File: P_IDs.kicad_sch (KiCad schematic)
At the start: 1 part

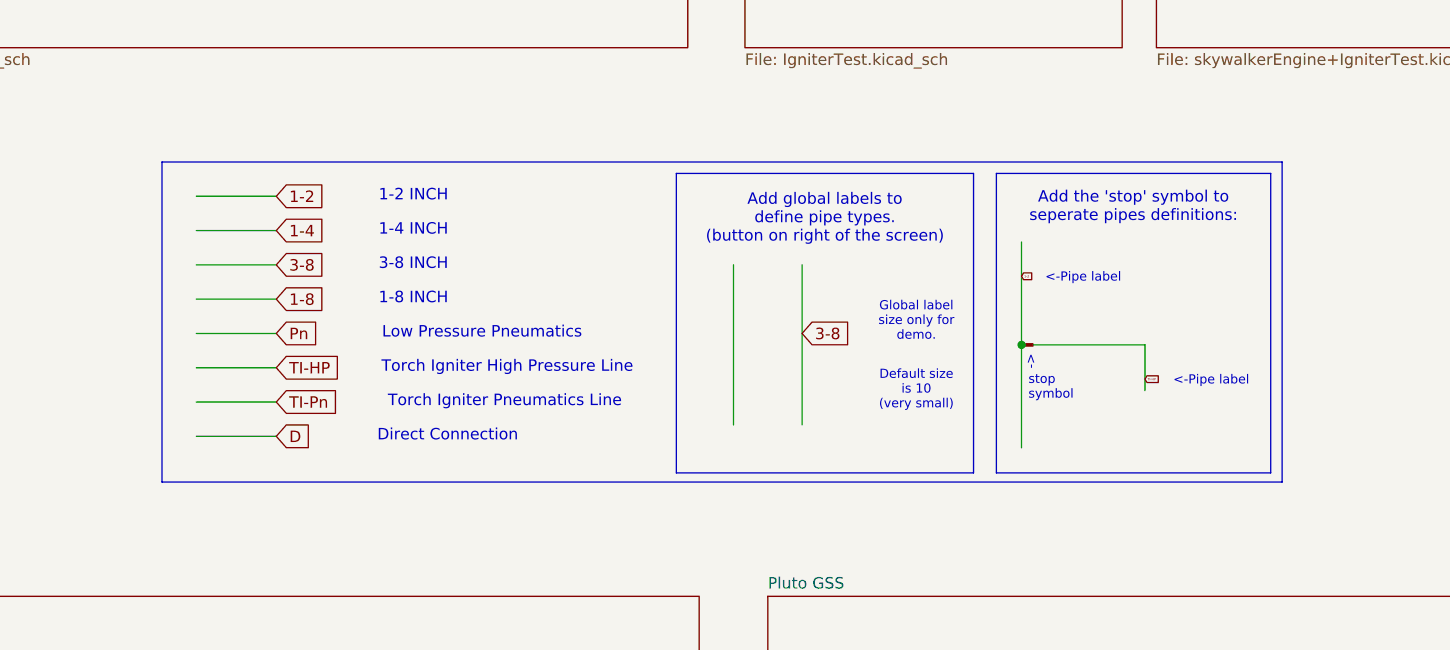
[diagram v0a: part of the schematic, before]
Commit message: bored
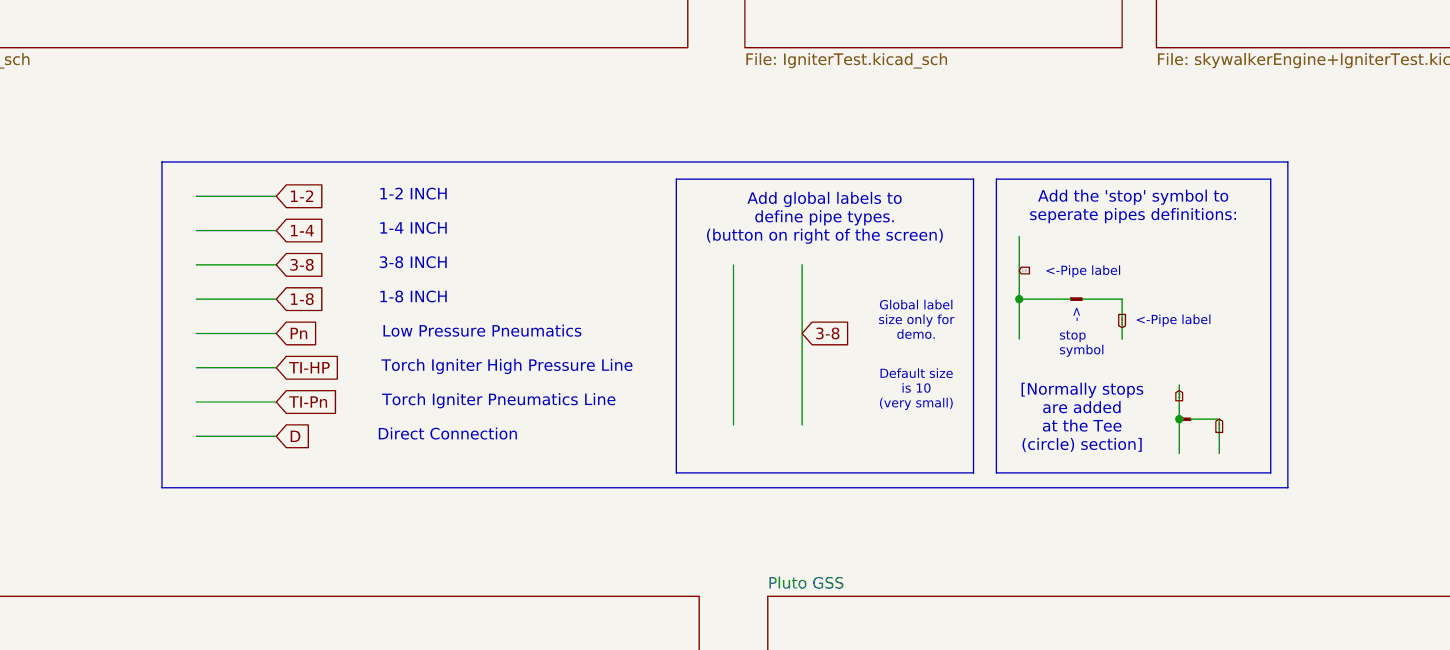
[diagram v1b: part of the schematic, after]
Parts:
- added U11: ~, symbol PID_symbols:stop
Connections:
- net 1-2: now also U11.
- net TI-HP: now also U11.
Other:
- note added: "[Normally stops are added at the Tee (circle) section]"
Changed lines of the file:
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@@
 	(rectangle
 		(start 62.23 86.36)
-		(end 186.69 121.92)
+		(end 187.325 122.555)
 		(stroke
 			(width 0)
@@
 	)
 	(rectangle
-		(start 154.94 87.63)
+		(start 154.94 88.265)
 		(end 185.42 120.904)
 		(stroke
@@
 	)
 	(rectangle
-		(start 119.38 87.63)
+		(start 119.38 88.265)
 		(end 152.4 120.904)
 		(stroke
@@
 	(text "<-Pipe label\n"
 		(exclude_from_sim no)
-		(at 164.592 99.314 0)
+		(at 164.592 98.679 0)
 		(effects
 			(font
@@
 	(text "stop\nsymbol"
 		(exclude_from_sim no)
-		(at 158.496 111.506 0)
+		(at 161.925 106.68 0)
 		(effects
 			(font
@@
 	(text "<-Pipe label\n"
 		(exclude_from_sim no)
-		(at 178.816 110.744 0)
+		(at 174.625 104.14 0)
 		(effects
 			(font
@@
 	(text "Torch Igniter Pneumatics Line"
 		(exclude_from_sim no)
-		(at 100.33 113.03 0)
+		(at 99.695 113.03 0)
 		(effects
 			(font
@@
 		)
 	)
+	(text "[Normally stops \nare added\nat the Tee \n(circle) section]"
+		(exclude_from_sim no)
+		(at 164.465 114.935 0)
+		(effects
+			(font
+				(size 1.27 1.27)
+				(color 204 102 0 1)
+			)
+		)
+	)
 	(text "->"
 		(exclude_from_sim no)
-		(at 158.75 108.712 90)
+		(at 163.83 103.505 90)
 		(effects
 			(font
@@
 	)
 	(junction
-		(at 157.734 106.68)
+		(at 157.48 101.6)
 		(diameter 0)
 		(color 0 0 0 0)
 	)
-	(wire
-		(pts
-			(xy 159.004 106.68) (xy 171.45 106.68)
-		)
-		(stroke
-			(width 0)
-			(type default)
-		)
+	(junction
+		(at 175.26 114.935)
+		(diameter 0)
+		(color 0 0 0 0)
 	)
 	(wire
@@
 	(wire
 		(pts
-			(xy 157.734 95.25) (xy 157.734 106.68)
+			(xy 175.26 111.125) (xy 175.26 114.935)
+		)
+		(stroke
+			(width 0)
+			(type default)
+		)
+	)
+	(wire
+		(pts
+			(xy 175.26 114.935) (xy 175.26 118.745)
+		)
+		(stroke
+			(width 0)
+			(type default)
+		)
+	)
+	(wire
+		(pts
+			(xy 157.48 94.615) (xy 157.48 101.6)
+		)
+		(stroke
+			(width 0)
+			(type default)
+		)
+	)
+	(wire
+		(pts
+			(xy 157.48 101.6) (xy 163.195 101.6)
 		)
 		(stroke
@@
 	(wire
 		(pts
+			(xy 157.48 101.6) (xy 157.48 106.045)
+		)
+		(stroke
+			(width 0)
+			(type default)
+		)
+	)
+	(wire
+		(pts
 			(xy 66.04 109.22) (xy 74.93 109.22)
 		)
@@
 	(wire
 		(pts
+			(xy 179.705 114.935) (xy 179.705 118.745)
+		)
+		(stroke
+			(width 0)
+			(type default)
+		)
+	)
+	(wire
+		(pts
 			(xy 66.04 93.98) (xy 74.93 93.98)
 		)
@@
 	(wire
 		(pts
-			(xy 157.734 106.68) (xy 157.734 118.11)
+			(xy 164.465 101.6) (xy 168.91 101.6)
 		)
 		(stroke
@@
 	(wire
 		(pts
-			(xy 171.45 106.68) (xy 171.45 111.76)
+			(xy 168.91 101.6) (xy 168.91 106.045)
+		)
+		(stroke
+			(width 0)
+			(type default)
+		)
+	)
+	(wire
+		(pts
+			(xy 176.53 114.935) (xy 179.705 114.935)
 		)
 		(stroke
@@
 		)
 	)
+	(global_label "TI-HP"
+		(shape input)
+		(at 179.705 114.935 270)
+		(fields_autoplaced yes)
+		(effects
+			(font
+				(size 0.254 0.254)
+			)
+			(justify right)
+		)
+		(property "Intersheetrefs" "${INTERSHEET_REFS}"
+			(at 179.705 116.6817 90)
+			(effects
+				(font
+					(size 1.27 1.27)
+				)
+				(justify right)
+				(hide yes)
+			)
+		)
+	)
 	(global_label "3-8"
 		(shape input)
@@
 	(global_label "1-2"
 		(shape input)
-		(at 157.734 99.06 0)
+		(at 157.48 98.425 0)
 		(fields_autoplaced yes)
 		(effects
@@
 		)
 		(property "Intersheetrefs" "${INTERSHEET_REFS}"
-			(at 159.1299 99.06 0)
-			(effects
-				(font
-					(size 1.27 1.27)
-				)
-				(justify left)
+			(at 158.8759 98.425 0)
+			(effects
+				(font
+					(size 1.27 1.27)
+				)
+				(justify left)
+				(hide yes)
+			)
+		)
+	)
+	(global_label "1-2"
+		(shape input)
+		(at 175.26 111.76 270)
+		(fields_autoplaced yes)
+		(effects
+			(font
+				(size 0.254 0.254)
+			)
+			(justify right)
+		)
+		(property "Intersheetrefs" "${INTERSHEET_REFS}"
+			(at 175.26 113.1559 90)
+			(effects
+				(font
+					(size 1.27 1.27)
+				)
+				(justify right)
 				(hide yes)
 			)
@@
 	(global_label "TI-HP"
 		(shape input)
-		(at 171.45 110.49 0)
+		(at 168.91 104.775 90)
 		(fields_autoplaced yes)
 		(effects
@@
 		)
 		(property "Intersheetrefs" "${INTERSHEET_REFS}"
-			(at 173.1967 110.49 0)
+			(at 168.91 103.0283 90)
 			(effects
 				(font
@@
 	(symbol
 		(lib_id "PID_symbols:stop")
-		(at 159.004 106.68 0)
+		(at 164.465 101.6 0)
 		(unit 1)
 		(exclude_from_sim no)
@@
 		(fields_autoplaced yes)
 		(property "Reference" "U6"
-			(at 161.29 106.172 0)
+			(at 166.751 101.092 0)
 			(effects
 				(font
@@
 		)
 		(property "Value" "~"
-			(at 158.369 105.41 0)
+			(at 163.83 100.33 0)
 			(effects
 				(font
@@
 		)
 		(property "Footprint" ""
-			(at 159.004 106.68 0)
+			(at 164.465 101.6 0)
 			(effects
 				(font
@@
 		)
 		(property "Datasheet" ""
-			(at 159.004 106.68 0)
+			(at 164.465 101.6 0)
 			(effects
 				(font
@@
 		)
 		(property "Description" ""
-			(at 159.004 106.68 0)
+			(at 164.465 101.6 0)
 			(effects
 				(font
@@
 					(unit 1)
 				)
+			)
+		)
+	)
+	(symbol
+		(lib_name "stop_1")
+		(lib_id "PID_symbols:stop")
+		(at 176.53 114.935 0)
+		(unit 1)
+		(exclude_from_sim no)
+		(in_bom no)
+		(on_board no)
+		(dnp no)
+		(fields_autoplaced yes)
+		(property "Reference" "U11"
+			(at 178.816 114.427 0)
+			(effects
+				(font
+					(size 1.27 1.27)
+				)
+				(hide yes)
+			)
+		)
+		(property "Value" "~"
+			(at 175.895 113.665 0)
+			(effects
+				(font
+					(size 1.27 1.27)
+				)
+			)
+		)
+		(property "Footprint" ""
+			(at 176.53 114.935 0)
+			(effects
+				(font
+					(size 1.27 1.27)
+				)
+				(hide yes)
+			)
+		)
+		(property "Datasheet" ""
+			(at 176.53 114.935 0)
+			(effects
+				(font
+					(size 1.27 1.27)
+				)
+				(hide yes)
+			)
+		)
+		(property "Description" ""
+			(at 176.53 114.935 0)
+			(effects
+				(font
+					(size 1.27 1.27)
+				)
+				(hide yes)
+			)
+		)
+		(pin ""
+		)
+		(pin ""
+		)
+		(instances
+			(project ""
+				(path "/045f1f05-3134-4b6d-91b6-463031104f1e"
+					(reference "U11")
+					(unit 1)
+				)

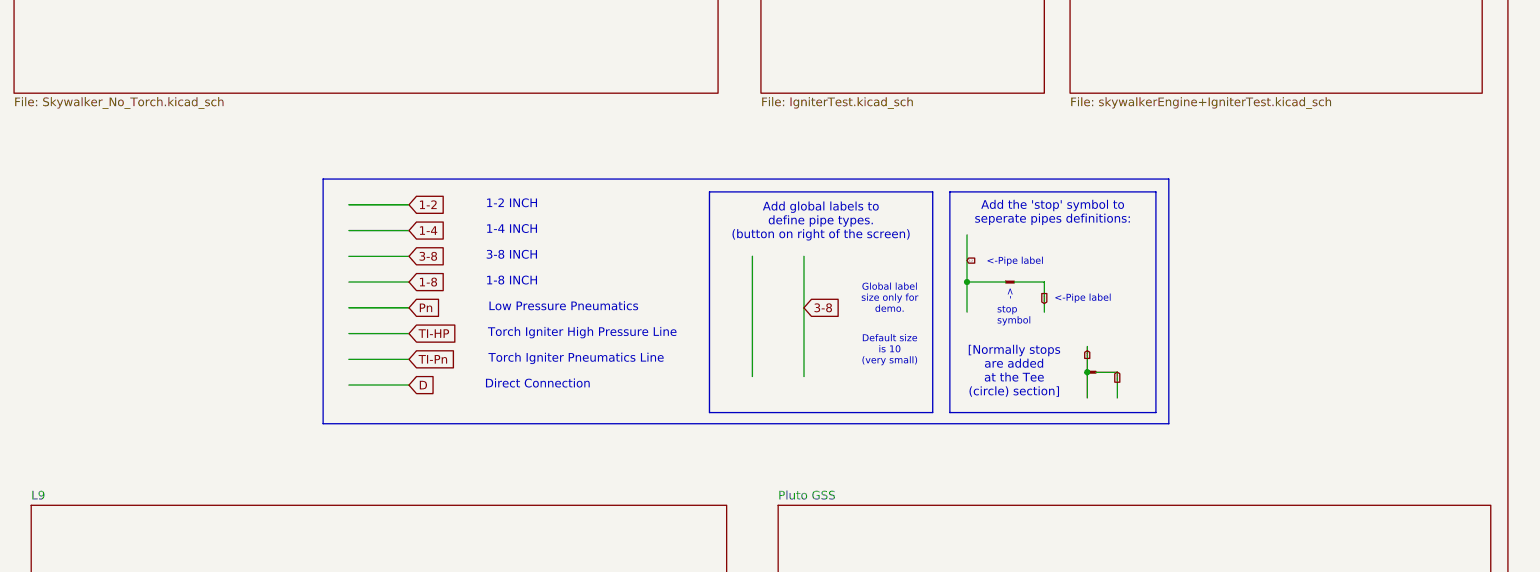
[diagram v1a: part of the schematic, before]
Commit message: Baboucarr Jeng
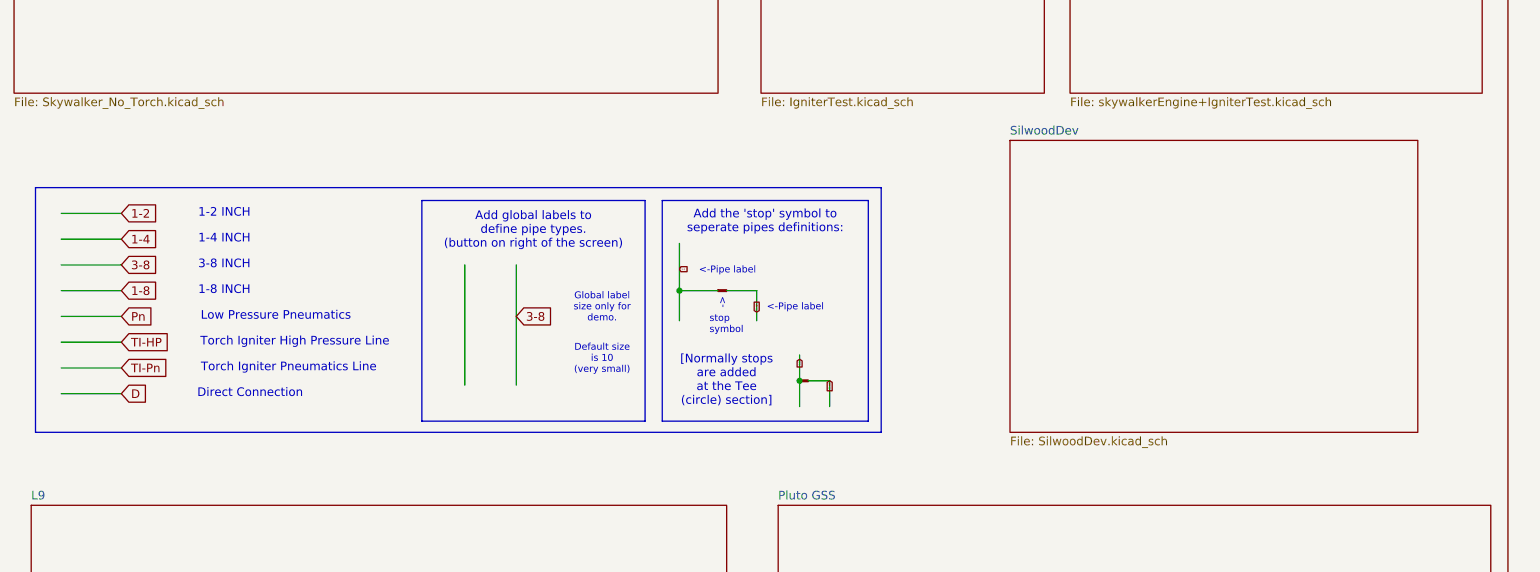
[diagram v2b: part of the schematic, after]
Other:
- added sheet SilwoodDev (SilwoodDev.kicad_sch)
